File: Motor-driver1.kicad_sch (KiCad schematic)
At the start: 32 parts, among them J8 PINHD_1x4_Male, J9 PINHD_1x4_Male, U2 DRV8825PWP, U3 DRV8825PWP

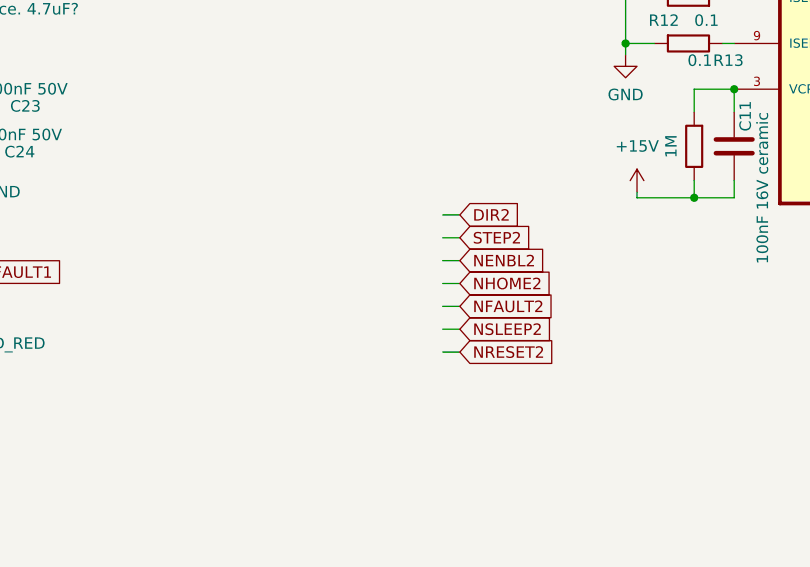
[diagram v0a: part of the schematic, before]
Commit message: last polishing on pcb v1. ich isch abgabe dc
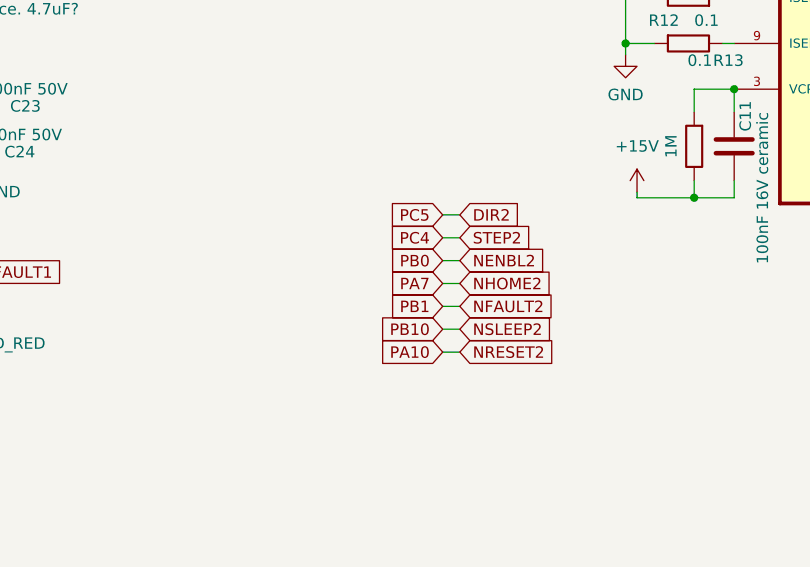
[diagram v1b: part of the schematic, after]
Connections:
- net STEP2 renamed PC4
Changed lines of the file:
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@@
+    )
+  )
+  (global_label "PA7" (shape input) (at 186.69 119.38 180) (fields_autoplaced)
+    (effects (font (size 1.27 1.27)) (justify right))
+    (property "Intersheetrefs" "${INTERSHEET_REFS}" (at 180.1367 119.38 0)
+      (effects (font (size 1.27 1.27)) (justify right) hide)
     )
   )
@@
     )
   )
+  (global_label "PC4" (shape input) (at 186.69 114.3 180) (fields_autoplaced)
+    (effects (font (size 1.27 1.27)) (justify right))
+    (property "Intersheetrefs" "${INTERSHEET_REFS}" (at 179.9553 114.3 0)
+      (effects (font (size 1.27 1.27)) (justify right) hide)
+    )
+  )
   (global_label "NSLEEP2" (shape input) (at 219.075 72.39 180) (fields_autoplaced)
     (effects (font (size 1.27 1.27)) (justify right))
@@
     )
   )
+  (global_label "PB10" (shape input) (at 186.69 124.46 180) (fields_autoplaced)
+    (effects (font (size 1.27 1.27)) (justify right))
+    (property "Intersheetrefs" "${INTERSHEET_REFS}" (at 178.7458 124.46 0)
+      (effects (font (size 1.27 1.27)) (justify right) hide)
+    )
+  )
   (global_label "PC3" (shape input) (at 46.355 61.595 180) (fields_autoplaced)
     (effects (font (size 1.27 1.27)) (justify right))
@@
     )
   )
+  (global_label "PB0" (shape input) (at 186.69 116.84 180) (fields_autoplaced)
+    (effects (font (size 1.27 1.27)) (justify right))
+    (property "Intersheetrefs" "${INTERSHEET_REFS}" (at 179.9553 116.84 0)
+      (effects (font (size 1.27 1.27)) (justify right) hide)
+    )
+  )
+  (global_label "PB1" (shape input) (at 186.69 121.92 180) (fields_autoplaced)
+    (effects (font (size 1.27 1.27)) (justify right))
+    (property "Intersheetrefs" "${INTERSHEET_REFS}" (at 179.9553 121.92 0)
+      (effects (font (size 1.27 1.27)) (justify right) hide)
+    )
+  )
   (global_label "NSLEEP1" (shape input) (at 125.095 128.905 270) (fields_autoplaced)
     (effects (font (size 1.27 1.27)) (justify right))
@@
     )
   )
+  (global_label "PC5" (shape input) (at 186.69 111.76 180) (fields_autoplaced)
+    (effects (font (size 1.27 1.27)) (justify right))
+    (property "Intersheetrefs" "${INTERSHEET_REFS}" (at 179.9553 111.76 0)
+      (effects (font (size 1.27 1.27)) (justify right) hide)
+    )
+  )
   (global_label "NSLEEP1" (shape input) (at 48.26 66.675 0) (fields_autoplaced)
     (effects (font (size 1.27 1.27)) (justify left))
@@
       (effects (font (size 1.27 1.27)) (justify right) hide)
     )
+  )
+  (global_label "PA10" (shape input) (at 186.69 127 180) (fields_autoplaced)
+    (effects (font (size 1.27 1.27)) (justify right))
+    (property "Intersheetrefs" "${INTERSHEET_REFS}" (at 178.9272 127 0)
+      (effects (font (size 1.27 1.27)) (justify right) hide)
+    )
